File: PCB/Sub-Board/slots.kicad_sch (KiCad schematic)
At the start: 119 parts, among them J10 Type, J11 Power/I2C, J12 Address, J13 Power/I2C, J14 Address, J15 GPIO, J16 Type, J17 GPIO, J18 Type, J19 Power/I2C, J20 Address, J21 Power/I2C, J22 Address, J23 GPIO, J24 Type, J25 GPIO, J26 Type, J27 Power/I2C, J28 Address, J29 Power/I2C, J3 Power/I2C, J30 Address, J31 GPIO, J32 Type, J33 GPIO, J34 Type, J4 Address, J5 Power/I2C, J6 Address, J7 GPIO, J8 Type, J9 GPIO

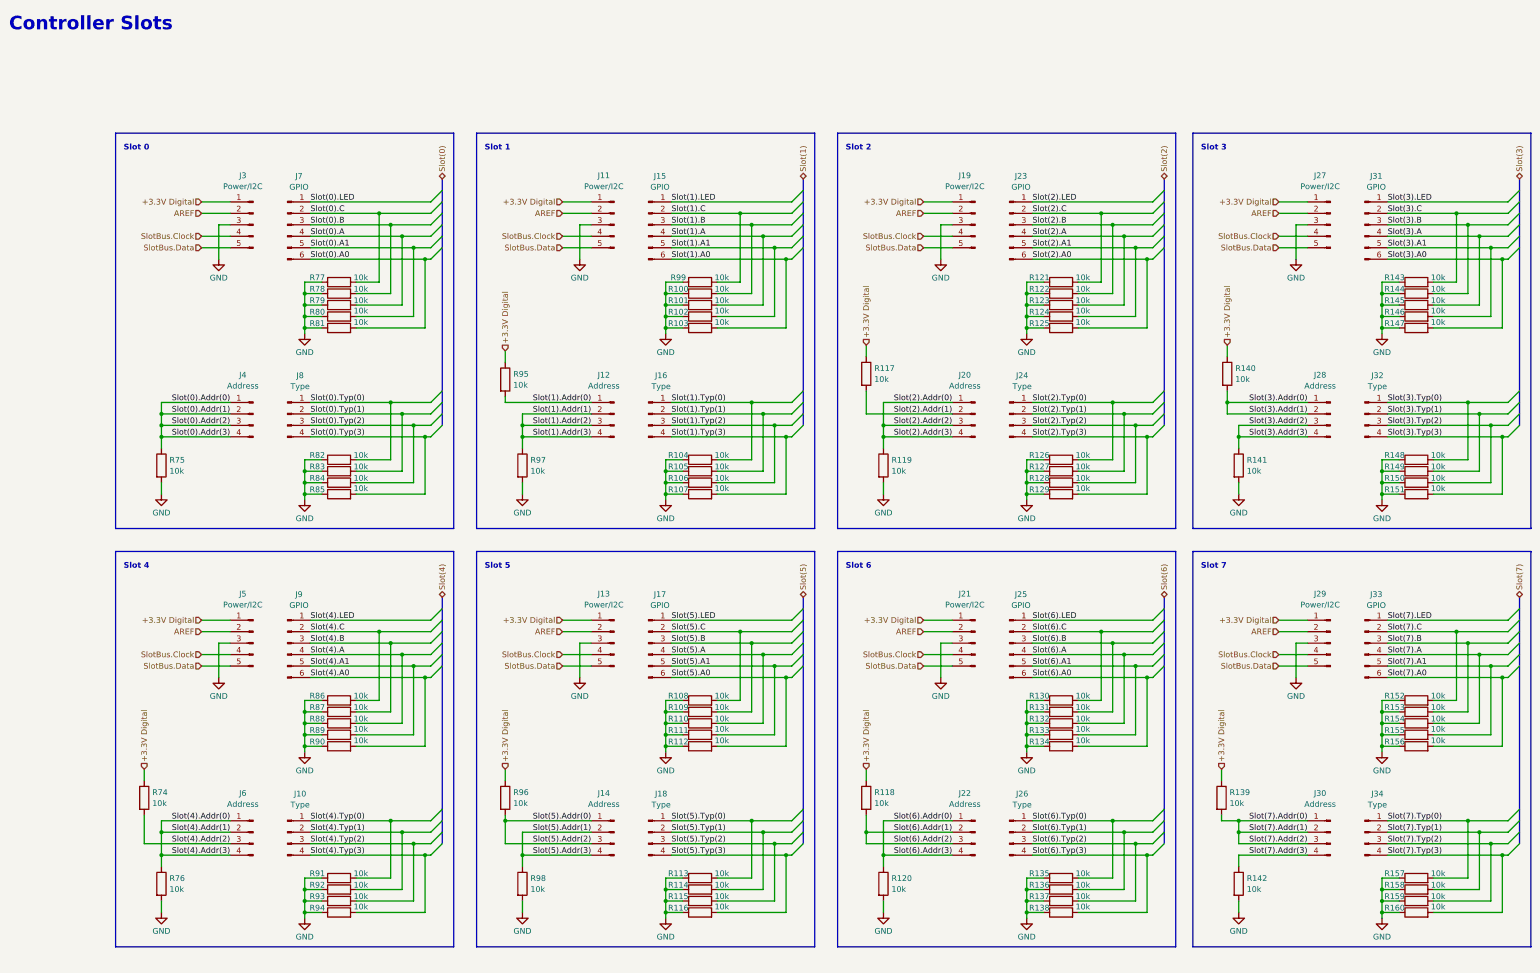
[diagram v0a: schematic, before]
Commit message: Sub-Board PCB after ERC
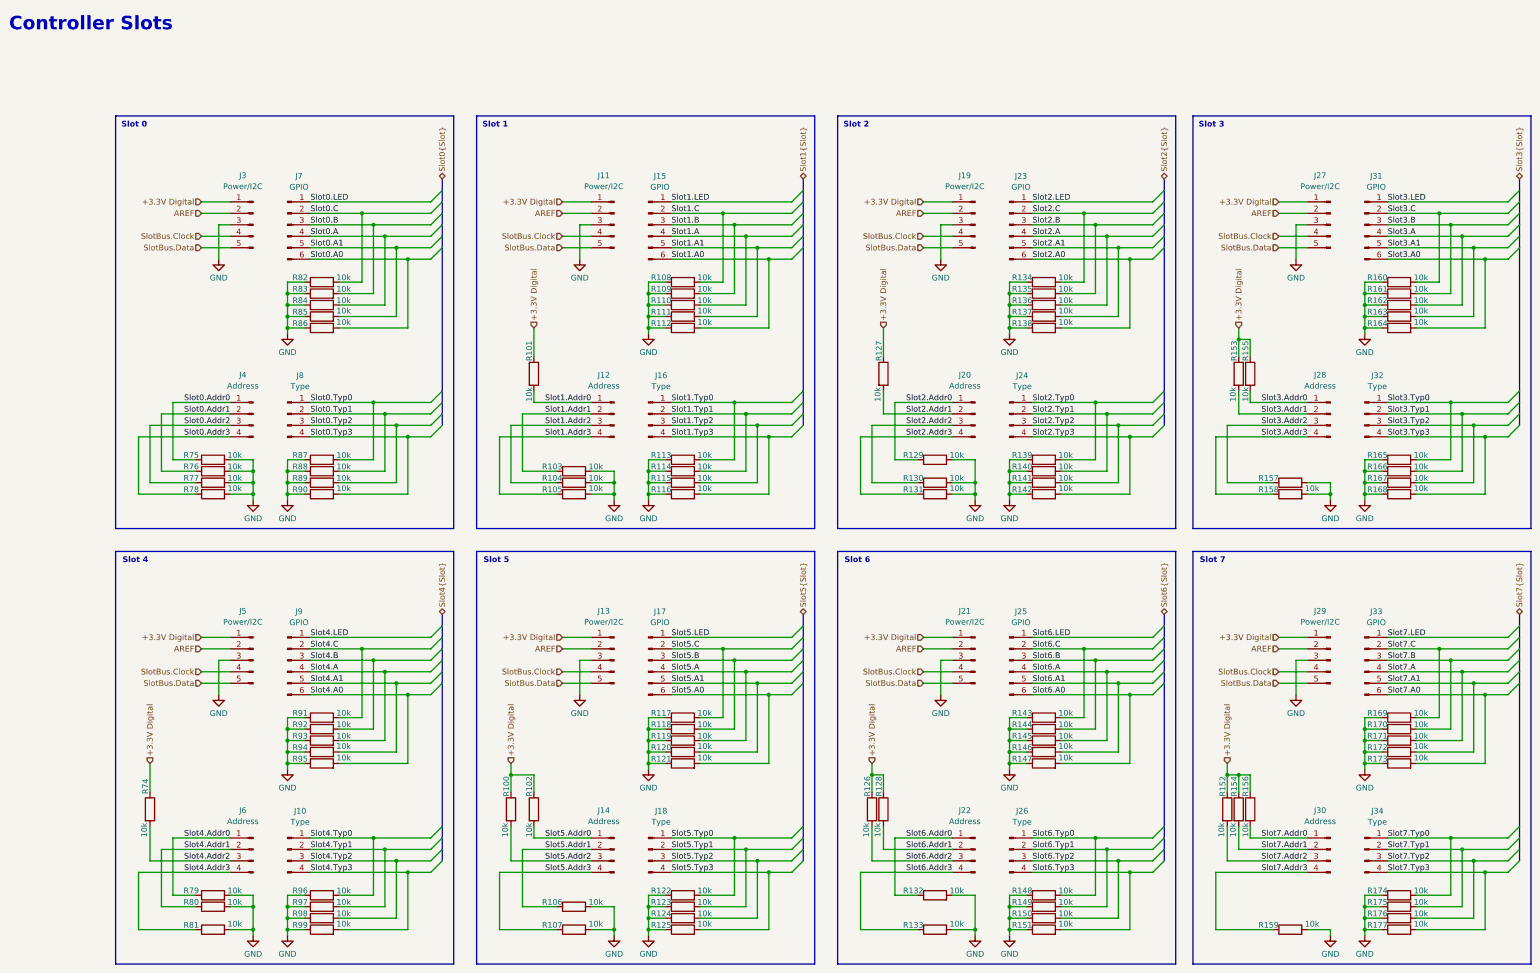
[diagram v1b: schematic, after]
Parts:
- removed R117, R118, R119, R120, R139, R140, R141, R142, R95, R96, R97, R98: 10k, symbol Device:R
- added R100, R101, R102, R103, R104, R105, R106, R107, R126, R127, R128, R129, R130, R131, R132, R133, R152, R153, R154, R155, R156, R157, R158, R159, R77, R78, R79, R80, R81: 10k, symbol Device:R
- renumbered R99 to R108, R100 to R109, R101 to R110, R102 to R111, R103 to R112, R104 to R113, R105 to R114, R106 to R115, R107 to R116, R108 to R117, R109 to R118, R110 to R119, R111 to R120, R112 to R121, R113 to R122, R114 to R123, R115 to R124, R116 to R125, R121 to R134, R122 to R135, R123 to R136, R124 to R137, R125 to R138, R126 to R139, R127 to R140, R128 to R141, R129 to R142, R130 to R143, R131 to R144, R132 to R145, R133 to R146, R134 to R147, R135 to R148, R136 to R149, R137 to R150, R138 to R151, R143 to R160, R144 to R161, R145 to R162, R146 to R163, R147 to R164, R148 to R165, R149 to R166, R150 to R167, R151 to R168, R152 to R169, R153 to R170, R154 to R171, R155 to R172, R156 to R173, R157 to R174, R158 to R175, R159 to R176, R160 to R177, R77 to R82, R78 to R83, R79 to R84, R80 to R85, R81 to R86, R82 to R87, R83 to R88, R84 to R89, R85 to R90, R86 to R91, R87 to R92, R88 to R93, R89 to R94, R90 to R95, R91 to R96, R92 to R97, R93 to R98, R94 to R99
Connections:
- net +3.3V Digital: now also R100.1, R101.1, R102.1, R126.1, R127.1, R128.1, R152.1, R153.1, R154.1, R155.1, R156.1
- net GND: now also R103.2, R104.2, R105.2, R106.2, R107.2, R129.2, R130.2, R131.2, R132.2, R133.2, R157.2, R158.2, R159.2, R77.2, R78.2, R79.2, R80.2, R81.2
- net Slot(0).A renamed Slot0.A
- net Slot(0).A0 renamed Slot0.A0
- net Slot(0).A1 renamed Slot0.A1
- removed net Slot(0).Addr(0): J4.1 (Pin_1), J4.2 (Pin_2), J4.3 (Pin_3), J4.4 (Pin_4), R75.1
- net Slot(0).B renamed Slot0.B
- net Slot(0).C renamed Slot0.C
- net Slot(0).LED renamed Slot0.LED
- net Slot(0).Typ(0) renamed Slot0.Typ0
- net Slot(0).Typ(1) renamed Slot0.Typ1
- net Slot(0).Typ(2) renamed Slot0.Typ2
- net Slot(0).Typ(3) renamed Slot0.Typ3
- net Slot(1).A renamed Slot1.A
- net Slot(1).A0 renamed Slot1.A0
- net Slot(1).A1 renamed Slot1.A1
- net Slot(1).Addr(0) renamed Slot1.Addr0
- net Slot1.Addr0: now also R101.2
- removed net Slot(1).Addr(1): J12.2 (Pin_2), J12.3 (Pin_3), J12.4 (Pin_4)
- net Slot(1).B renamed Slot1.B
- net Slot(1).C renamed Slot1.C
- net Slot(1).LED renamed Slot1.LED
- net Slot(1).Typ(0) renamed Slot1.Typ0
- net Slot(1).Typ(1) renamed Slot1.Typ1
- net Slot(1).Typ(2) renamed Slot1.Typ2
- net Slot(1).Typ(3) renamed Slot1.Typ3
- net Slot(2).A renamed Slot2.A
- net Slot(2).A0 renamed Slot2.A0
- net Slot(2).A1 renamed Slot2.A1
- removed net Slot(2).Addr(0): J20.1 (Pin_1), J20.3 (Pin_3), J20.4 (Pin_4)
- net Slot(2).Addr(1) renamed Slot2.Addr1
- net Slot2.Addr1: now also R127.2
- net Slot(2).B renamed Slot2.B
- net Slot(2).C renamed Slot2.C
- net Slot(2).LED renamed Slot2.LED
- net Slot(2).Typ(0) renamed Slot2.Typ0
- net Slot(2).Typ(1) renamed Slot2.Typ1
- net Slot(2).Typ(2) renamed Slot2.Typ2
- net Slot(2).Typ(3) renamed Slot2.Typ3
- net Slot(3).A renamed Slot3.A
- net Slot(3).A0 renamed Slot3.A0
- net Slot(3).A1 renamed Slot3.A1
- net Slot(3).Addr(0) renamed Slot3.Addr0
- net Slot3.Addr0: now also R155.2; no longer J28.2 (Pin_2)
- net Slot(3).Addr(2) renamed Slot3.Addr2
- net Slot3.Addr2: now also R157.1; no longer J28.4 (Pin_4)
- net Slot(3).B renamed Slot3.B
- net Slot(3).C renamed Slot3.C
- net Slot(3).LED renamed Slot3.LED
- net Slot(3).Typ(0) renamed Slot3.Typ0
- net Slot(3).Typ(1) renamed Slot3.Typ1
- net Slot(3).Typ(2) renamed Slot3.Typ2
- net Slot(3).Typ(3) renamed Slot3.Typ3
- net Slot(4).A renamed Slot4.A
- net Slot(4).A0 renamed Slot4.A0
- net Slot(4).A1 renamed Slot4.A1
- removed net Slot(4).Addr(0): J6.1 (Pin_1), J6.2 (Pin_2), J6.4 (Pin_4), R76.1
- net Slot(4).Addr(2) renamed Slot4.Addr2
- net Slot(4).B renamed Slot4.B
- net Slot(4).C renamed Slot4.C
- net Slot(4).LED renamed Slot4.LED
- net Slot(4).Typ(0) renamed Slot4.Typ0
- net Slot(4).Typ(1) renamed Slot4.Typ1
- net Slot(4).Typ(2) renamed Slot4.Typ2
- net Slot(4).Typ(3) renamed Slot4.Typ3
- net Slot(5).A renamed Slot5.A
- net Slot(5).A0 renamed Slot5.A0
- net Slot(5).A1 renamed Slot5.A1
- net Slot(5).Addr(0) renamed Slot5.Addr0
- net Slot5.Addr0: now also R102.2; no longer J14.3 (Pin_3)
- net Slot(5).Addr(1) renamed Slot5.Addr1
- net Slot5.Addr1: now also R106.1; no longer J14.4 (Pin_4)
- net Slot(5).B renamed Slot5.B
- net Slot(5).C renamed Slot5.C
- net Slot(5).LED renamed Slot5.LED
- net Slot(5).Typ(0) renamed Slot5.Typ0
- net Slot(5).Typ(1) renamed Slot5.Typ1
- net Slot(5).Typ(2) renamed Slot5.Typ2
- net Slot(5).Typ(3) renamed Slot5.Typ3
- net Slot(6).A renamed Slot6.A
- net Slot(6).A0 renamed Slot6.A0
- net Slot(6).A1 renamed Slot6.A1
- net Slot(6).Addr(0) renamed Slot6.Addr0
- net Slot6.Addr0: now also R132.1; no longer J22.4 (Pin_4)
- net Slot(6).Addr(1) renamed Slot6.Addr1
- net Slot6.Addr1: now also R128.2; no longer J22.3 (Pin_3)
- net Slot(6).B renamed Slot6.B
- net Slot(6).C renamed Slot6.C
- net Slot(6).LED renamed Slot6.LED
- net Slot(6).Typ(0) renamed Slot6.Typ0
- net Slot(6).Typ(1) renamed Slot6.Typ1
- net Slot(6).Typ(2) renamed Slot6.Typ2
- net Slot(6).Typ(3) renamed Slot6.Typ3
- net Slot(7).A renamed Slot7.A
- net Slot(7).A0 renamed Slot7.A0
- net Slot(7).A1 renamed Slot7.A1
- removed net Slot(7).Addr(0): J30.1 (Pin_1), J30.2 (Pin_2), J30.3 (Pin_3)
- net Slot(7).Addr(3) renamed Slot7.Addr3
- net Slot7.Addr3: now also R159.1
- net Slot(7).B renamed Slot7.B
- net Slot(7).C renamed Slot7.C
- net Slot(7).LED renamed Slot7.LED
- net Slot(7).Typ(0) renamed Slot7.Typ0
- net Slot(7).Typ(1) renamed Slot7.Typ1
- net Slot(7).Typ(2) renamed Slot7.Typ2
- net Slot(7).Typ(3) renamed Slot7.Typ3
- new net Slot0.Addr0: J4.1 (Pin_1), R75.1
- new net Slot0.Addr1: J4.2 (Pin_2), R76.1
- new net Slot0.Addr2: J4.3 (Pin_3), R77.1
- new net Slot0.Addr3: J4.4 (Pin_4), R78.1
- new net Slot1.Addr1: J12.2 (Pin_2), R103.1
- new net Slot1.Addr2: J12.3 (Pin_3), R104.1
- new net Slot1.Addr3: J12.4 (Pin_4), R105.1
- new net Slot2.Addr0: J20.1 (Pin_1), R129.1
- new net Slot2.Addr2: J20.3 (Pin_3), R130.1
- new net Slot2.Addr3: J20.4 (Pin_4), R131.1
- new net Slot3.Addr1: J28.2 (Pin_2), R153.2
- new net Slot3.Addr3: J28.4 (Pin_4), R158.1
- new net Slot4.Addr0: J6.1 (Pin_1), R79.1
- new net Slot4.Addr1: J6.2 (Pin_2), R80.1
- new net Slot4.Addr3: J6.4 (Pin_4), R81.1
- new net Slot5.Addr2: J14.3 (Pin_3), R100.2
- new net Slot5.Addr3: J14.4 (Pin_4), R107.1
- new net Slot6.Addr2: J22.3 (Pin_3), R126.2
- new net Slot6.Addr3: J22.4 (Pin_4), R133.1
- new net Slot7.Addr0: J30.1 (Pin_1), R156.2
- new net Slot7.Addr1: J30.2 (Pin_2), R154.2
- new net Slot7.Addr2: J30.3 (Pin_3), R152.2
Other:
- moved on the sheet: J10, J13, J14, J17, J18, J21, J22, J25, J26, J29, J30, J33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
